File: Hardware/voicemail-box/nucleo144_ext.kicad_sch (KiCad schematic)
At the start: 3 parts, among them J401 Micro_SD_Card_Det1

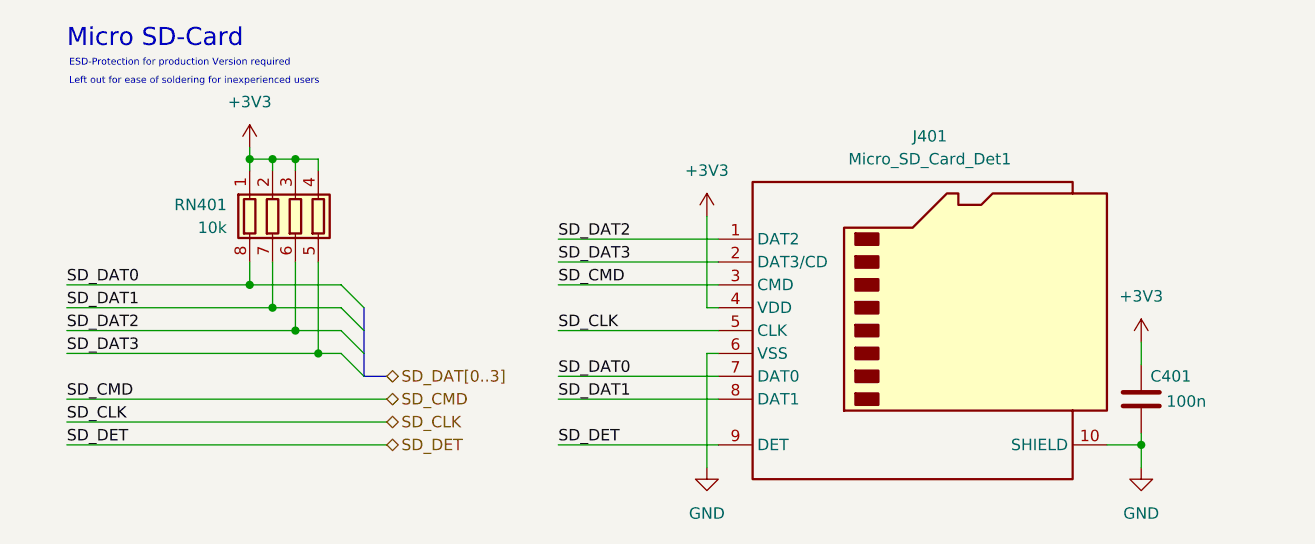
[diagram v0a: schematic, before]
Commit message: ~layout
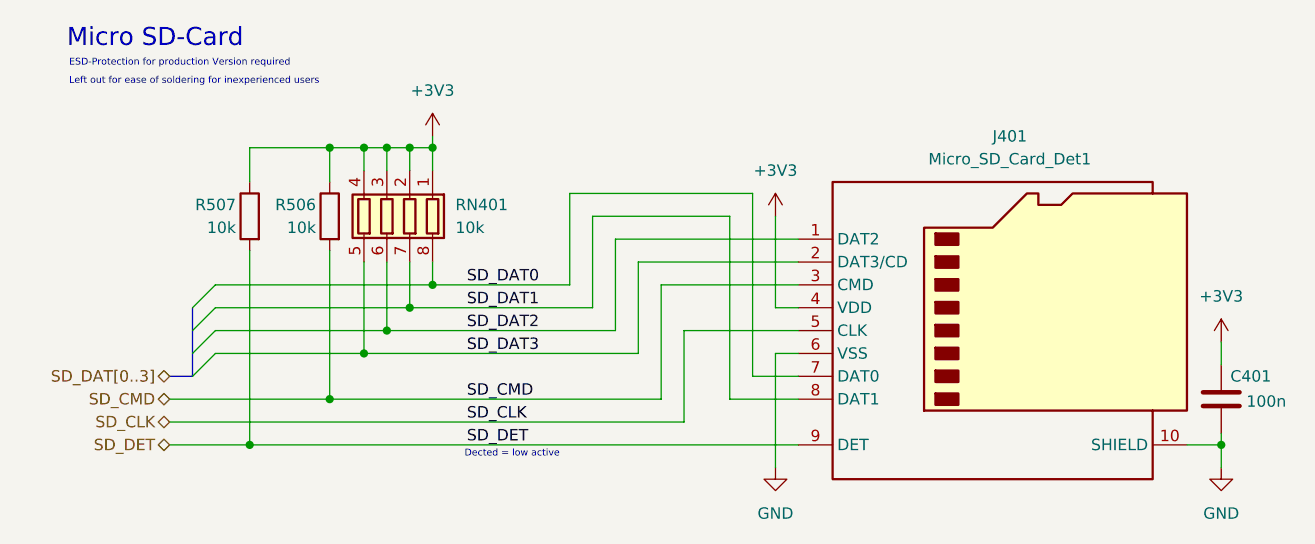
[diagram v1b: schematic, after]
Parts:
- added R506, R507: 10k, Resistor_SMD:R_0805_2012Metric_Pad1.20x1.40mm_HandSolder, symbol Device:R
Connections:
- net +3V3: now also R506.1, R507.1
- net SD_CMD: now also R506.2
- net SD_DET: now also R507.2
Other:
- note added: "Dected = low active"
- moved on the sheet: C401, J401, RN401
